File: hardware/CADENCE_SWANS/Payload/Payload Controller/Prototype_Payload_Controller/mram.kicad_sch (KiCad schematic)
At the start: 3 parts

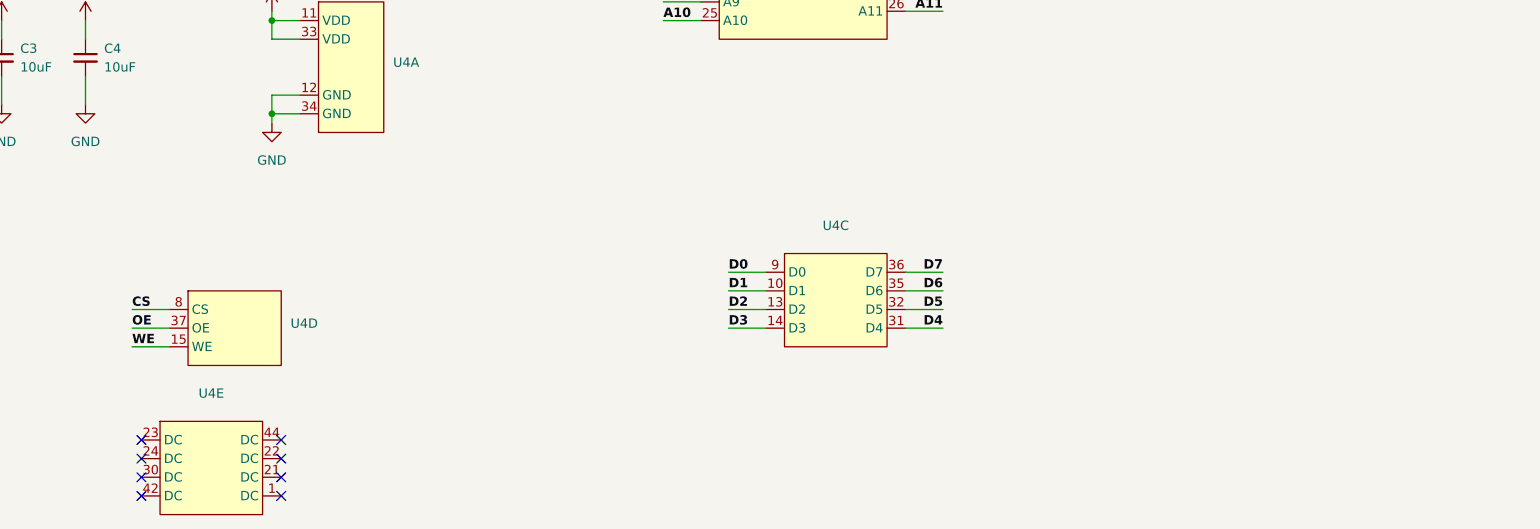
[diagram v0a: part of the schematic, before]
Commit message: updates
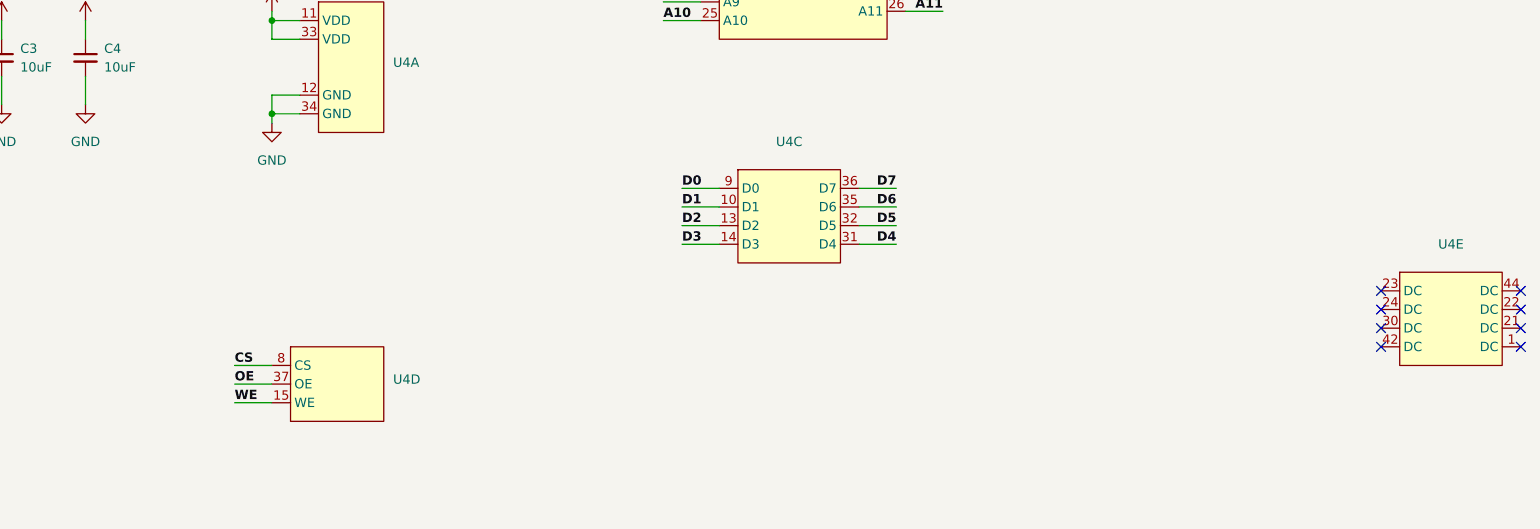
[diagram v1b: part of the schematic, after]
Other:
- moved on the sheet: U4C, U4D, U4E
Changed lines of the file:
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@@
 	)
 	(no_connect
-		(at 69.85 163.83)
+		(at 238.76 143.51)
 	)
 	(no_connect
-		(at 88.9 163.83)
+		(at 257.81 143.51)
 	)
 	(no_connect
-		(at 69.85 156.21)
+		(at 238.76 135.89)
 	)
 	(no_connect
-		(at 69.85 158.75)
+		(at 238.76 138.43)
 	)
 	(no_connect
-		(at 88.9 156.21)
+		(at 257.81 135.89)
 	)
 	(no_connect
-		(at 69.85 161.29)
+		(at 238.76 140.97)
 	)
 	(no_connect
-		(at 88.9 161.29)
+		(at 257.81 140.97)
 	)
 	(no_connect
-		(at 88.9 158.75)
+		(at 257.81 138.43)
 	)
 	(bus_entry
@@
 	(wire
 		(pts
-			(xy 173.99 135.89) (xy 179.07 135.89)
+			(xy 167.64 124.46) (xy 172.72 124.46)
 		)
 		(stroke
@@
 	(wire
 		(pts
-			(xy 68.58 138.43) (xy 73.66 138.43)
+			(xy 82.55 146.05) (xy 87.63 146.05)
 		)
 		(stroke
@@
 	(wire
 		(pts
-			(xy 68.58 140.97) (xy 73.66 140.97)
+			(xy 82.55 148.59) (xy 87.63 148.59)
 		)
 		(stroke
@@
 	(wire
 		(pts
-			(xy 68.58 143.51) (xy 73.66 143.51)
+			(xy 82.55 151.13) (xy 87.63 151.13)
 		)
 		(stroke
@@
 	(wire
 		(pts
-			(xy 149.86 138.43) (xy 154.94 138.43)
+			(xy 143.51 127) (xy 148.59 127)
 		)
 		(stroke
@@
 	(wire
 		(pts
-			(xy 149.86 135.89) (xy 154.94 135.89)
+			(xy 143.51 124.46) (xy 148.59 124.46)
 		)
 		(stroke
@@
 	(wire
 		(pts
-			(xy 173.99 140.97) (xy 179.07 140.97)
+			(xy 167.64 129.54) (xy 172.72 129.54)
 		)
 		(stroke
@@
 	(wire
 		(pts
-			(xy 173.99 133.35) (xy 179.07 133.35)
+			(xy 167.64 121.92) (xy 172.72 121.92)
 		)
 		(stroke
@@
 	(wire
 		(pts
-			(xy 173.99 138.43) (xy 179.07 138.43)
+			(xy 167.64 127) (xy 172.72 127)
 		)
 		(stroke
@@
 	(wire
 		(pts
-			(xy 149.86 133.35) (xy 154.94 133.35)
+			(xy 143.51 121.92) (xy 148.59 121.92)
 		)
 		(stroke
@@
 	(wire
 		(pts
-			(xy 149.86 140.97) (xy 154.94 140.97)
+			(xy 143.51 129.54) (xy 148.59 129.54)
 		)
 		(stroke
@@
 	)
 	(label "D0"
-		(at 149.86 133.35 0)
+		(at 143.51 121.92 0)
 		(effects
 			(font
@@
 	)
 	(label "D5"
-		(at 179.07 138.43 180)
+		(at 172.72 127 180)
 		(effects
 			(font
@@
 	)
 	(label "OE"
-		(at 68.58 140.97 0)
+		(at 82.55 148.59 0)
 		(effects
 			(font
@@
 	)
 	(label "D6"
-		(at 179.07 135.89 180)
+		(at 172.72 124.46 180)
 		(effects
 			(font
@@
 	)
 	(label "D7"
-		(at 179.07 133.35 180)
+		(at 172.72 121.92 180)
 		(effects
 			(font
@@
 	)
 	(label "WE"
-		(at 68.58 143.51 0)
+		(at 82.55 151.13 0)
 		(effects
 			(font
@@
 	)
 	(label "D3"
-		(at 149.86 140.97 0)
+		(at 143.51 129.54 0)
 		(effects
 			(font
@@
 	)
 	(label "D1"
-		(at 149.86 135.89 0)
+		(at 143.51 124.46 0)
 		(effects
 			(font
@@
 	)
 	(label "D2"
-		(at 149.86 138.43 0)
+		(at 143.51 127 0)
 		(effects
 			(font
@@
 	)
 	(label "D4"
-		(at 179.07 140.97 180)
+		(at 172.72 129.54 180)
 		(effects
 			(font
@@
 	)
 	(label "CS"
-		(at 68.58 138.43 0)
+		(at 82.55 146.05 0)
 		(effects
 			(font
@@
 	(symbol
 		(lib_id "Payload_Controller_EM:MR4A08B")
-		(at 76.2 146.05 0)
+		(at 90.17 153.67 0)
 		(unit 4)
 		(exclude_from_sim no)
@@
 		(fields_autoplaced yes)
 		(property "Reference" "U4"
-			(at 90.17 140.3349 0)
+			(at 104.14 147.9549 0)
 			(effects
 				(font
@@
 		)
 		(property "Value" "~"
-			(at 90.17 142.24 0)
+			(at 104.14 149.86 0)
 			(effects
 				(font
@@
 		)
 		(property "Footprint" ""
-			(at 76.2 146.05 0)
+			(at 90.17 153.67 0)
 			(effects
 				(font
@@
 		)
 		(property "Datasheet" ""
-			(at 76.2 146.05 0)
+			(at 90.17 153.67 0)
 			(effects
 				(font
@@
 		)
 		(property "Description" ""
-			(at 76.2 146.05 0)
+			(at 90.17 153.67 0)
 			(effects
 				(font
@@
 	(symbol
 		(lib_id "Payload_Controller_EM:MR4A08B")
-		(at 157.48 143.51 0)
+		(at 151.13 132.08 0)
 		(unit 3)
 		(exclude_from_sim no)
@@
 		(fields_autoplaced yes)
 		(property "Reference" "U4"
-			(at 164.465 127 0)
+			(at 158.115 115.57 0)
 			(effects
 				(font
@@
 		)
 		(property "Value" "~"
-			(at 164.465 129.54 0)
+			(at 158.115 118.11 0)
 			(effects
 				(font
@@
 		)
 		(property "Footprint" ""
-			(at 157.48 143.51 0)
+			(at 151.13 132.08 0)
 			(effects
 				(font
@@
 		)
 		(property "Datasheet" ""
-			(at 157.48 143.51 0)
+			(at 151.13 132.08 0)
 			(effects
 				(font
@@
 		)
 		(property "Description" ""
-			(at 157.48 143.51 0)
+			(at 151.13 132.08 0)
 			(effects
 				(font
@@
 	(symbol
 		(lib_id "Payload_Controller_EM:MR4A08B")
-		(at 72.39 166.37 0)
+		(at 241.3 146.05 0)
 		(unit 5)
 		(exclude_from_sim no)
@@
 		(fields_autoplaced yes)
 		(property "Reference" "U4"
-			(at 79.375 149.86 0)
+			(at 248.285 129.54 0)
 			(effects
 				(font
@@
 		)
 		(property "Value" "~"
-			(at 79.375 152.4 0)
+			(at 248.285 132.08 0)
 			(effects
 				(font
@@
 		)
 		(property "Footprint" ""
-			(at 72.39 166.37 0)
+			(at 241.3 146.05 0)
 			(effects
 				(font
@@
 		)
 		(property "Datasheet" ""
-			(at 72.39 166.37 0)
+			(at 241.3 146.05 0)
 			(effects
 				(font
@@
 		)
 		(property "Description" ""
-			(at 72.39 166.37 0)
+			(at 241.3 146.05 0)
 			(effects
 				(font
